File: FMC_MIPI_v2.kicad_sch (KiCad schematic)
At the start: 0 parts

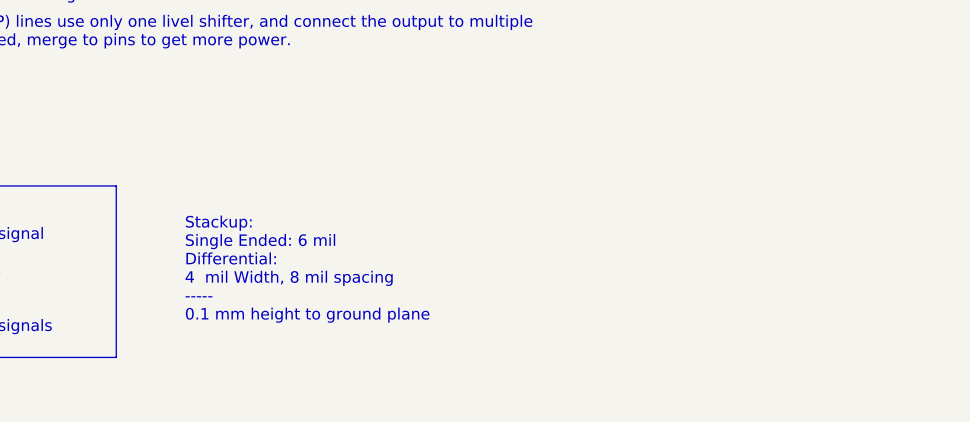
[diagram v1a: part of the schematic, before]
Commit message: JLCPCB BOM OK
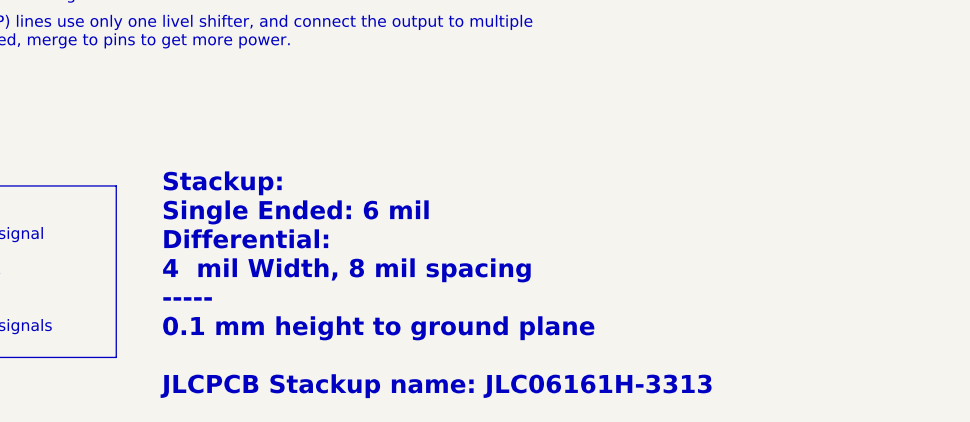
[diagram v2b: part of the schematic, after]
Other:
- note added: "Stackup: Single Ended: 6 mil Differential: 4 mil Width, 8 mil spacing ----- 0.1 mm height to ground plane JLCPCB Stackup name: JLC06161H-3313"
- note removed: "Stackup: Single Ended: 6 mil Differential: 4 mil Width, 8 mil spacing ----- 0.1 mm height to ground plane"
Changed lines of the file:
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@@
     (effects (font (size 1.27 1.27)) (justify left bottom))
   )
-  (text "Stackup:\nSingle Ended: 6 mil\nDifferential:\n4  mil Width, 8 mil spacing\n-----\n0.1 mm height to ground plane\n"
-    (at 58.42 154.94 0)
-    (effects (font (size 1.27 1.27)) (justify left bottom))
+  (text "Stackup:\nSingle Ended: 6 mil\nDifferential:\n4  mil Width, 8 mil spacing\n-----\n0.1 mm height to ground plane\n\nJLCPCB Stackup name: JLC06161H-3313\n"
+    (at 55.88 163.195 0)
+    (effects (font (size 2 2) (thickness 0.254) bold) (justify left bottom))
   )
   (label "VOLT_3P3" (at 54.61 29.21 0)
@@
     )
     (path "/00000000-0000-0000-0000-000061aca102/00000000-0000-0000-0000-0000637a2fc5"
-      (reference "R29") (unit 1) (value "1k") (footprint "Resistors_SMD:R_0805")
+      (reference "R29") (unit 1) (value "2.2k") (footprint "Resistors_SMD:R_0805")
     )
     (path "/00000000-0000-0000-0000-000061aca102/00000000-0000-0000-0000-00006376ce9d"
@@
     )
     (path "/00000000-0000-0000-0000-00006362ecc5/00000000-0000-0000-0000-0000638632db"
-      (reference "R31") (unit 1) (value "1k") (footprint "Resistors_SMD:R_0805")
+      (reference "R31") (unit 1) (value "2.2k") (footprint "Resistors_SMD:R_0805")
     )
     (path "/00000000-0000-0000-0000-000061aca102/00000000-0000-0000-0000-0000638d5ec5"
-      (reference "R32") (unit 1) (value "1k") (footprint "Resistors_SMD:R_0805")
+      (reference "R32") (unit 1) (value "2.2k") (footprint "Resistors_SMD:R_0805")
     )
     (path "/00000000-0000-0000-0000-000061aca102/00000000-0000-0000-0000-0000638d5eb1"
@@
     )
     (path "/00000000-0000-0000-0000-000061aca102/00000000-0000-0000-0000-000063a1f4ee"
-      (reference "R34") (unit 1) (value "1k") (footprint "Resistors_SMD:R_0805")
+      (reference "R34") (unit 1) (value "2.2k") (footprint "Resistors_SMD:R_0805")
     )
     (path "/00000000-0000-0000-0000-00006362ecc5/00000000-0000-0000-0000-000063b3066e"
@@
     )
     (path "/00000000-0000-0000-0000-00006362ecc5/00000000-0000-0000-0000-000063673675"
-      (reference "U3") (unit 1) (value "SN74AVCH16T245_DGV_48") (footprint "FMC_MIPI_v2_sym:DGV48")
+      (reference "U3") (unit 1) (value "SN74AVCH16T245GR") (footprint "FMC_MIPI_v2_sym:SOP50P810X120-48N")
     )
     (path "/00000000-0000-0000-0000-0000637747ef/00000000-0000-0000-0000-00006379d961"
@@
     )
     (path "/00000000-0000-0000-0000-00006191d89c/00000000-0000-0000-0000-0000636800c7"
-      (reference "U8") (unit 1) (value "SN74AVCH16T245_DGV_48") (footprint "FMC_MIPI_v2_sym:DGV48")
-    )
-  )
+      (reference "U8") (unit 1) (value "SN74AVCH16T245GR") (footprint "FMC_MIPI_v2_sym:SOP50P810X120-48N")
+    )
+  )
